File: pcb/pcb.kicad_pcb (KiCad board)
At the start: 2 copper layers, 0 parts

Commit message: Add files via upload
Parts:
- added 3.3vconverter1: ATA00F18S-L, Converter_DCDC:Converter_DCDC_Artesyn_ATA_SMD, F.Cu at (173.4, 101.6)
- added 5Vconverter1: ATA00A18S-L, Converter_DCDC:Converter_DCDC_Artesyn_ATA_SMD, F.Cu at (137.8, 121.9)
- added BT1: Battery, Connector_AMASS:AMASS_XT60-F_1x02_P7.20mm_Vertical, F.Cu at (153.4, 119.5)
- added BT2: Battery, Connector_AMASS:AMASS_XT30U-F_1x02_P5.0mm_Vertical, F.Cu at (151.9, 128.2)
- added BZ1: Buzzer, custom:buzer, F.Cu at (180.1, 118.2)
- added R1: R, custom:resistor, F.Cu at (169.6, 125.7)
- added R2: R, custom:resistor, F.Cu at (152.6, 146.1)
- added R3: R, custom:resistor, F.Cu at (157.7, 143.5)
- added R4: R, custom:resistor, F.Cu at (152.6, 148.6)
- added R5: R, custom:resistor, F.Cu at (180.1, 120.7)
- added R6: R, custom:resistor, F.Cu at (167.8, 133.2)
- added R7: R, custom:resistor, F.Cu at (160.2, 140.7)
- added collor_sensor_1: tcs3472_color_sensor, custom:tcs3472, F.Cu at (112.0, 129.8)
- added collor_sensor_2: tcs3472_color_sensor, custom:tcs3472, F.Cu at (112.0, 134.3)
- added collor_sensor_3: tcs3472_color_sensor, custom:tcs3472, F.Cu at (112.0, 138.9)
- added collor_sensor_4: tcs3472_color_sensor, custom:tcs3472, F.Cu at (129.8, 138.5)
- added collor_sensor_5: tcs3472_color_sensor, custom:tcs3472, F.Cu at (112.0, 143.4)
- added collor_sensor_6: tcs3472_color_sensor, custom:tcs3472, F.Cu at (112.0, 148.0)
- added controllboard1: Teensy4.1, custom:teensy4.1, F.Cu at (96.8, 97.7)
- added i2converter1: PCA9548ADB, Package_SO:SSOP-24_5.3x8.2mm_P0.65mm, F.Cu at (171.1, 119.4)
- added io_expender2: MCP23017_SP, Package_DIP:DIP-28_W7.62mm, F.Cu at (107.3, 90.9)
- added io_expernder1: MCP23017_SP, Package_DIP:DIP-28_W7.62mm, F.Cu at (118.2, 90.9)
- added ir_sensor_1: tssp4038, custom:tssp4038, F.Cu at (142.5, 143.5)
- added ir_sensor_10: tssp4038, custom:tssp4038, F.Cu at (187.6, 105.3)
- added ir_sensor_11: tssp4038, custom:tssp4038, F.Cu at (160.2, 135.7)
- added ir_sensor_12: tssp4038, custom:tssp4038, F.Cu at (187.6, 107.8)
- added ir_sensor_13: tssp4038, custom:tssp4038, F.Cu at (167.8, 128.2)
- added ir_sensor_14: tssp4038, custom:tssp4038, F.Cu at (187.6, 110.3)
- added ir_sensor_15: tssp4038, custom:tssp4038, F.Cu at (160.2, 138.2)
- added ir_sensor_16: tssp4038, custom:tssp4038, F.Cu at (187.6, 112.9)
- added ir_sensor_2: tssp4038, custom:tssp4038, F.Cu at (180.1, 115.6)
- added ir_sensor_3: tssp4038, custom:tssp4038, F.Cu at (145.0, 148.6)
- added ir_sensor_4: tssp4038, custom:tssp4038, F.Cu at (150.1, 143.5)
- added ir_sensor_5: tssp4038, custom:tssp4038, F.Cu at (145.0, 146.1)
- added ir_sensor_6: tssp4038, custom:tssp4038, F.Cu at (160.2, 133.1)
- added ir_sensor_7: tssp4038, custom:tssp4038, F.Cu at (137.4, 148.1)
- added ir_sensor_8: tssp4038, custom:tssp4038, F.Cu at (152.0, 133.1)
- added ir_sensor_9: tssp4038, custom:tssp4038, F.Cu at (167.8, 130.7)
- added motor1: pololu_motor, custom:pololu_motor, F.Cu at (129.8, 148.1)
- added motor2: pololu_motor, custom:pololu_motor, F.Cu at (154.6, 112.9)
- added motor3: pololu_motor, custom:pololu_motor, F.Cu at (154.6, 110.4)
- added motor_driver1: l298n, custom:l298n, F.Cu at (129.8, 140.5)
- added motor_driver2: l298n, custom:l298n, F.Cu at (147.6, 135.9)
- added openmvcam1: openMV_M7_R2, custom:openmv_m7_r2, F.Cu at (145.2, 96.4)
- added set_goal_color1: SW_DIP_x01, custom:dipswitch1, F.Cu at (187.7, 115.4)
- added settings1: SW_DIP_x06, custom:dipswitch6, F.Cu at (187.6, 95.2)

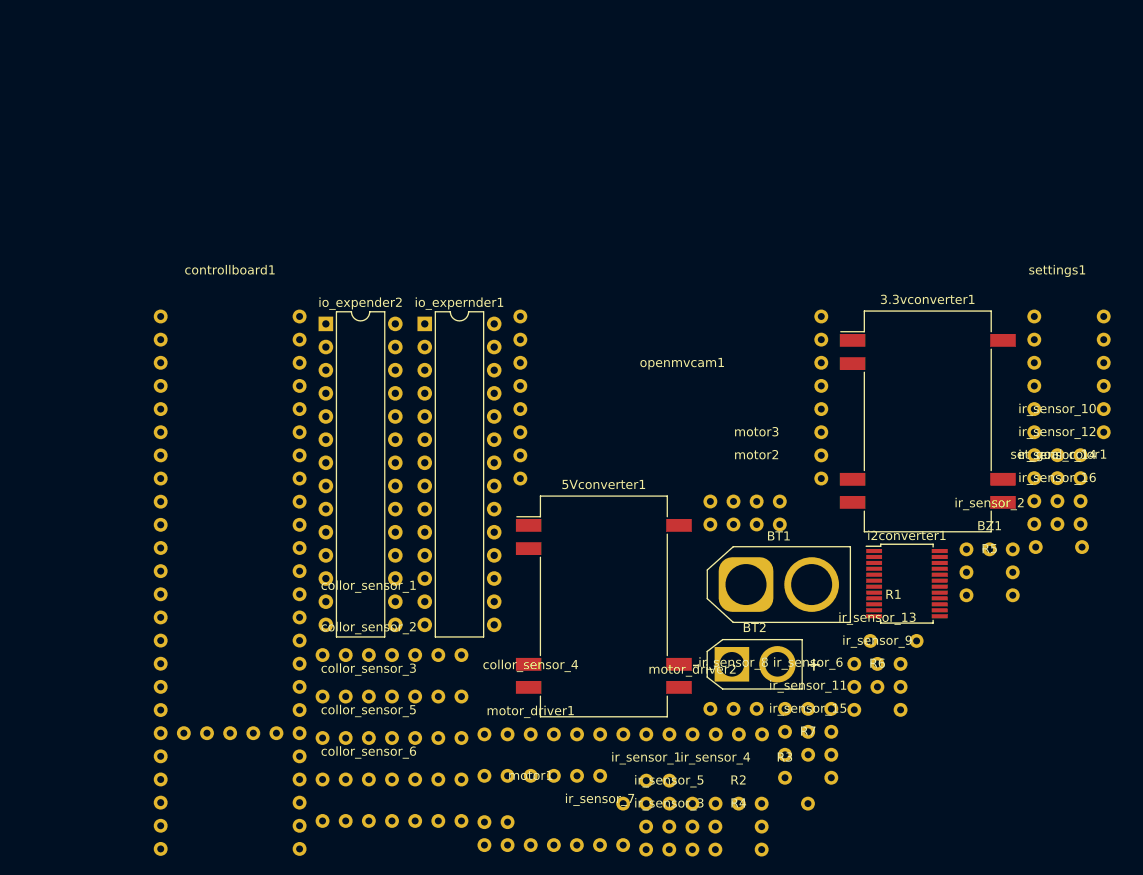
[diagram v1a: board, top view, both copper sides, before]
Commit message: Commit message
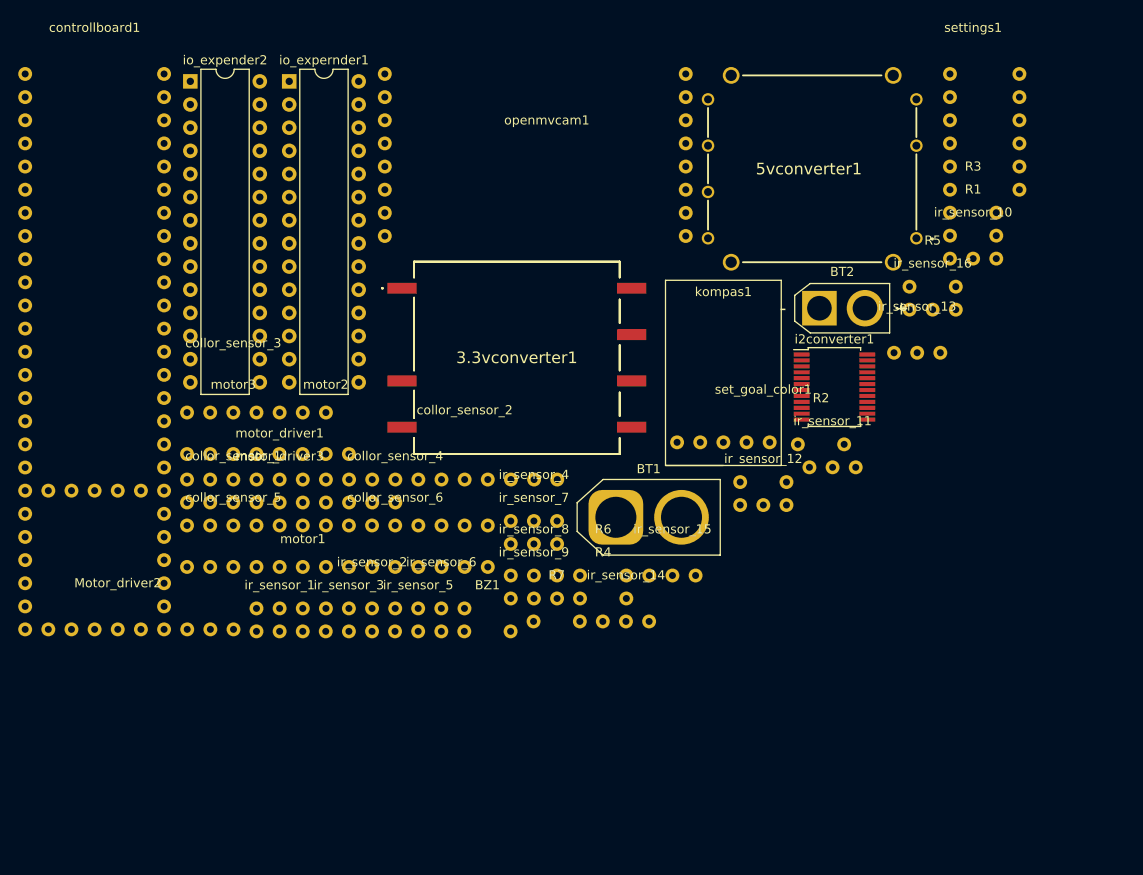
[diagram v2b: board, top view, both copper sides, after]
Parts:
- removed 5Vconverter1: ATA00A18S-L, Converter_DCDC:Converter_DCDC_Artesyn_ATA_SMD
- removed motor_driver2: l298n, custom:l298n
- added 5vconverter1: CC6-1205SF-E, custom:CC6_SF, F.Cu at (149.2, 68.8)
- added Motor_driver2: TB9051FTG, custom:TB9051FTG, F.Cu at (84.5, 124.4)
- added kompas1: miniIMU-9_v6, custom:miniIMU-9_v6, F.Cu at (150.9, 93.7)
- added motor_driver3: TB9051FTG, custom:TB9051FTG, F.Cu at (102.2, 110.5)
- 3.3vconverter1: value ATA00F18S-L -> CC6-1203SR-E; footprint Converter_DCDC:Converter_DCDC_Artesyn_ATA_SMD -> custom:CC60512SRE
- motor_driver1: value l298n -> TB9051FTG; footprint custom:l298n -> custom:TB9051FTG
- moved ir_sensor_2 68.1 mm to (112.4, 122.1)
- moved R3 68.1 mm to (178.3, 78.7)
- moved motor3 57.7 mm to (97.2, 105.2)
- moved BZ1 55.5 mm to (125.0, 124.6)
- moved ir_sensor_14 49.1 mm to (140.2, 123.5)
- moved motor2 47.9 mm to (107.3, 105.2)
- moved 3.3vconverter1 45.6 mm to (128.3, 94.6)
- moved R1 45.3 mm to (178.3, 81.2)
- moved ir_sensor_1 44.4 mm to (102.2, 124.6)
- moved R2 42.9 mm to (161.6, 104.1)
- moved motor_driver1 42.6 mm to (102.2, 108.0)
- moved ir_sensor_3 42.5 mm to (109.8, 124.6)
- moved ir_sensor_6 41.7 mm to (120.0, 122.1)
- moved BT2 40.2 mm to (161.5, 89.2)
- moved ir_sensor_9 38.9 mm to (130.1, 121.0)
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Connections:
- 3.3vconverter1 pad 1: gnd -> 12v
- BZ1 pad 2: Net-(5Vconverter1-Pad10) -> Net-(5vconverter1-Pad5)
- R1 pad 2: Net-(3.3vconverter1-Pad10) -> Net-(3.3vconverter1-Pad5)
- R2 pad 2: Net-(5Vconverter1-Pad10) -> Net-(5vconverter1-Pad5)
- R3 pad 2: Net-(5Vconverter1-Pad10) -> Net-(5vconverter1-Pad5)
- R4 pad 2: Net-(5Vconverter1-Pad10) -> Net-(5vconverter1-Pad5)
- R5 pad 2: Net-(5Vconverter1-Pad10) -> Net-(5vconverter1-Pad5)
- R6 pad 2: Net-(5Vconverter1-Pad10) -> Net-(5vconverter1-Pad5)
- R7 pad 2: Net-(5Vconverter1-Pad10) -> Net-(5vconverter1-Pad5)
- collor_sensor_1 pad 2: Net-(3.3vconverter1-Pad9) -> Net-(3.3vconverter1-Pad7)
- collor_sensor_1 pad 3: Net-(3.3vconverter1-Pad10) -> Net-(3.3vconverter1-Pad5)
- collor_sensor_2 pad 2: Net-(3.3vconverter1-Pad9) -> Net-(3.3vconverter1-Pad7)
- collor_sensor_2 pad 3: Net-(3.3vconverter1-Pad10) -> Net-(3.3vconverter1-Pad5)
- collor_sensor_3 pad 2: Net-(3.3vconverter1-Pad9) -> Net-(3.3vconverter1-Pad7)
- collor_sensor_3 pad 3: Net-(3.3vconverter1-Pad10) -> Net-(3.3vconverter1-Pad5)
- collor_sensor_4 pad 2: Net-(3.3vconverter1-Pad9) -> Net-(3.3vconverter1-Pad7)
- collor_sensor_4 pad 3: Net-(3.3vconverter1-Pad10) -> Net-(3.3vconverter1-Pad5)
- collor_sensor_5 pad 2: Net-(3.3vconverter1-Pad9) -> Net-(3.3vconverter1-Pad7)
- collor_sensor_5 pad 3: Net-(3.3vconverter1-Pad10) -> Net-(3.3vconverter1-Pad5)
- collor_sensor_6 pad 2: Net-(3.3vconverter1-Pad9) -> Net-(3.3vconverter1-Pad7)
- collor_sensor_6 pad 3: Net-(3.3vconverter1-Pad10) -> Net-(3.3vconverter1-Pad5)
- controllboard1 pad 47: Net-(5Vconverter1-Pad10) -> Net-(5vconverter1-Pad5)
- controllboard1 pad 48: Net-(5Vconverter1-Pad9) -> Net-(5vconverter1-Pad7)
- i2converter1 pad 12: Net-(3.3vconverter1-Pad10) -> Net-(3.3vconverter1-Pad5)
- i2converter1 pad 24: Net-(3.3vconverter1-Pad9) -> Net-(3.3vconverter1-Pad7)
- io_expender2 pad 10: Net-(3.3vconverter1-Pad10) -> Net-(3.3vconverter1-Pad5)
- io_expender2 pad 2: Net-(io_expender2-Pad2) -> Net-(Motor_driver2-Pad12)
- io_expender2 pad 3: Net-(io_expender2-Pad3) -> Net-(Motor_driver2-Pad11)
- io_expender2 pad 4: Net-(io_expender2-Pad4) -> Net-(Motor_driver2-Pad10)
- io_expender2 pad 5: Net-(io_expender2-Pad5) -> Net-(Motor_driver2-Pad9)
- io_expender2 pad 9: Net-(3.3vconverter1-Pad9) -> Net-(3.3vconverter1-Pad7)
- io_expernder1 pad 10: Net-(3.3vconverter1-Pad10) -> Net-(3.3vconverter1-Pad5)
- io_expernder1 pad 9: Net-(3.3vconverter1-Pad9) -> Net-(3.3vconverter1-Pad7)
- ir_sensor_1 pad 1: Net-(3.3vconverter1-Pad9) -> Net-(3.3vconverter1-Pad7)
- ir_sensor_1 pad 2: Net-(3.3vconverter1-Pad10) -> Net-(3.3vconverter1-Pad5)
- ir_sensor_10 pad 1: Net-(3.3vconverter1-Pad9) -> Net-(3.3vconverter1-Pad7)
- ir_sensor_10 pad 2: Net-(3.3vconverter1-Pad10) -> Net-(3.3vconverter1-Pad5)
- ir_sensor_11 pad 1: Net-(3.3vconverter1-Pad9) -> Net-(3.3vconverter1-Pad7)
- ir_sensor_11 pad 2: Net-(3.3vconverter1-Pad10) -> Net-(3.3vconverter1-Pad5)
- ir_sensor_12 pad 1: Net-(3.3vconverter1-Pad9) -> Net-(3.3vconverter1-Pad7)
- ir_sensor_12 pad 2: Net-(3.3vconverter1-Pad10) -> Net-(3.3vconverter1-Pad5)
- ir_sensor_13 pad 1: Net-(3.3vconverter1-Pad9) -> Net-(3.3vconverter1-Pad7)
- ir_sensor_13 pad 2: Net-(3.3vconverter1-Pad10) -> Net-(3.3vconverter1-Pad5)
- ir_sensor_14 pad 1: Net-(3.3vconverter1-Pad9) -> Net-(3.3vconverter1-Pad7)
- ir_sensor_14 pad 2: Net-(3.3vconverter1-Pad10) -> Net-(3.3vconverter1-Pad5)
- ir_sensor_15 pad 1: Net-(3.3vconverter1-Pad9) -> Net-(3.3vconverter1-Pad7)
- ir_sensor_15 pad 2: Net-(3.3vconverter1-Pad10) -> Net-(3.3vconverter1-Pad5)
- ir_sensor_16 pad 1: Net-(3.3vconverter1-Pad9) -> Net-(3.3vconverter1-Pad7)
- ir_sensor_16 pad 2: Net-(3.3vconverter1-Pad10) -> Net-(3.3vconverter1-Pad5)
- ir_sensor_2 pad 1: Net-(3.3vconverter1-Pad9) -> Net-(3.3vconverter1-Pad7)
- ir_sensor_2 pad 2: Net-(3.3vconverter1-Pad10) -> Net-(3.3vconverter1-Pad5)
- ir_sensor_3 pad 1: Net-(3.3vconverter1-Pad9) -> Net-(3.3vconverter1-Pad7)
- ir_sensor_3 pad 2: Net-(3.3vconverter1-Pad10) -> Net-(3.3vconverter1-Pad5)
- ir_sensor_4 pad 1: Net-(3.3vconverter1-Pad9) -> Net-(3.3vconverter1-Pad7)
- ir_sensor_4 pad 2: Net-(3.3vconverter1-Pad10) -> Net-(3.3vconverter1-Pad5)
- ir_sensor_5 pad 1: Net-(3.3vconverter1-Pad9) -> Net-(3.3vconverter1-Pad7)
- ir_sensor_5 pad 2: Net-(3.3vconverter1-Pad10) -> Net-(3.3vconverter1-Pad5)
- ir_sensor_6 pad 1: Net-(3.3vconverter1-Pad9) -> Net-(3.3vconverter1-Pad7)
- ir_sensor_6 pad 2: Net-(3.3vconverter1-Pad10) -> Net-(3.3vconverter1-Pad5)
- ir_sensor_7 pad 1: Net-(3.3vconverter1-Pad9) -> Net-(3.3vconverter1-Pad7)
- ir_sensor_7 pad 2: Net-(3.3vconverter1-Pad10) -> Net-(3.3vconverter1-Pad5)
- ir_sensor_8 pad 1: Net-(3.3vconverter1-Pad9) -> Net-(3.3vconverter1-Pad7)
- ir_sensor_8 pad 2: Net-(3.3vconverter1-Pad10) -> Net-(3.3vconverter1-Pad5)
- ir_sensor_9 pad 1: Net-(3.3vconverter1-Pad9) -> Net-(3.3vconverter1-Pad7)
- ir_sensor_9 pad 2: Net-(3.3vconverter1-Pad10) -> Net-(3.3vconverter1-Pad5)
- motor1 pad 1: Net-(5Vconverter1-Pad9) -> Net-(5vconverter1-Pad7)
- motor1 pad 4: Net-(5Vconverter1-Pad10) -> Net-(5vconverter1-Pad5)
- motor2 pad 1: Net-(5Vconverter1-Pad9) -> Net-(5vconverter1-Pad7)
- motor2 pad 4: Net-(5Vconverter1-Pad10) -> Net-(5vconverter1-Pad5)
- motor3 pad 1: Net-(5Vconverter1-Pad9) -> Net-(5vconverter1-Pad7)
- motor3 pad 4: Net-(5Vconverter1-Pad10) -> Net-(5vconverter1-Pad5)
- motor_driver1 pad 10: Net-(io_expender2-Pad6) -> Net-(io_expender2-Pad8)
- motor_driver1 pad 5: Net-(io_expender2-Pad1) -> Net-(motor_driver1-Pad5)
- motor_driver1 pad 6: Net-(io_expender2-Pad2) -> Net-(5vconverter1-Pad5)
- motor_driver1 pad 7: Net-(io_expender2-Pad3) -> Net-(5vconverter1-Pad7)
- motor_driver1 pad 8: Net-(io_expender2-Pad4) -> Net-(motor_driver1-Pad8)
- motor_driver1 pad 9: Net-(io_expender2-Pad5) -> Net-(io_expender2-Pad21)
- set_goal_color1 pad 1: Net-(3.3vconverter1-Pad9) -> Net-(3.3vconverter1-Pad7)
